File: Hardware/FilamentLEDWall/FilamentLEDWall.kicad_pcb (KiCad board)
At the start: 2 copper layers, 23 parts, among them U1 AMS1117-3.3, U2 AMS1117-5.0, U3 JXI5020GF

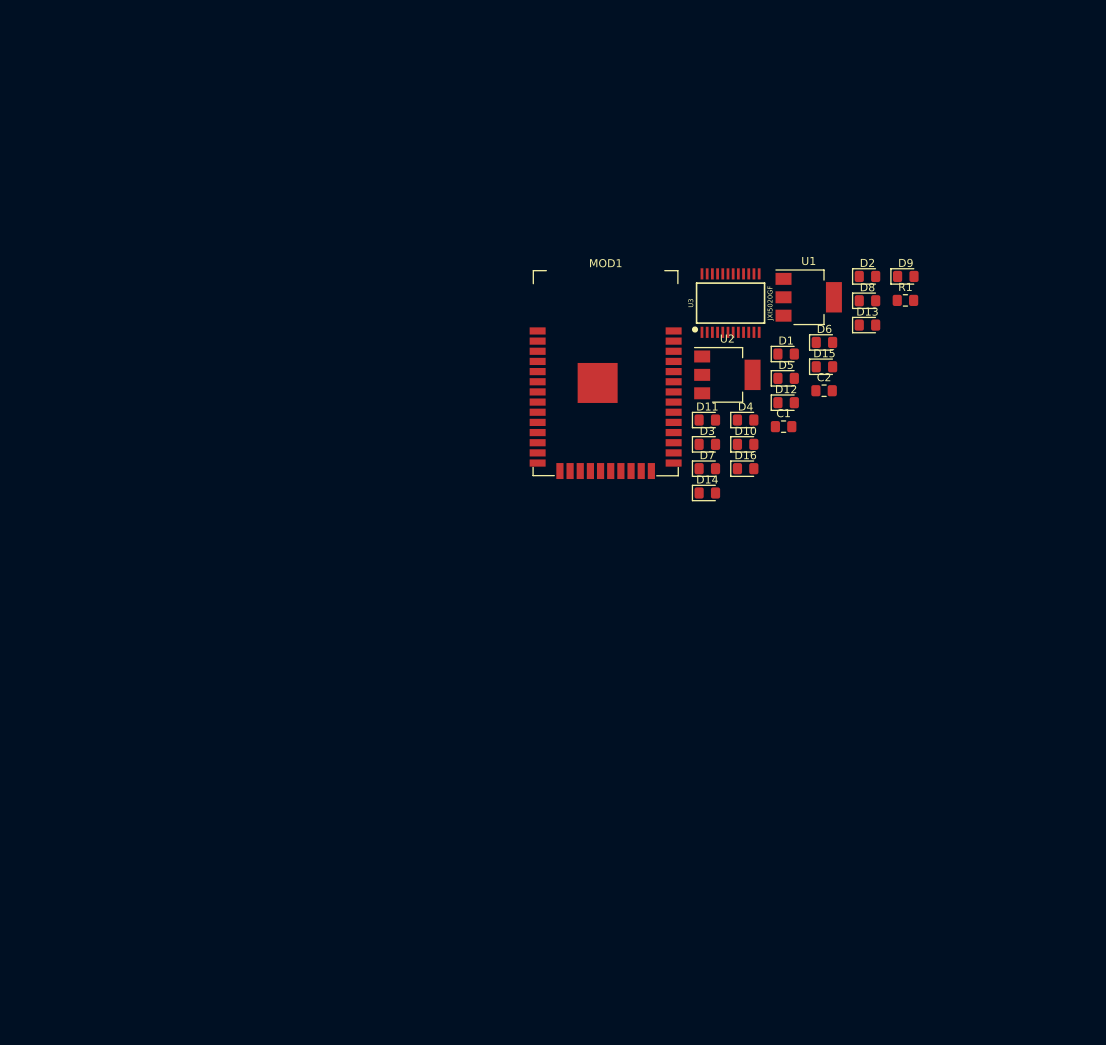
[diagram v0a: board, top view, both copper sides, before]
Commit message: updated circuit
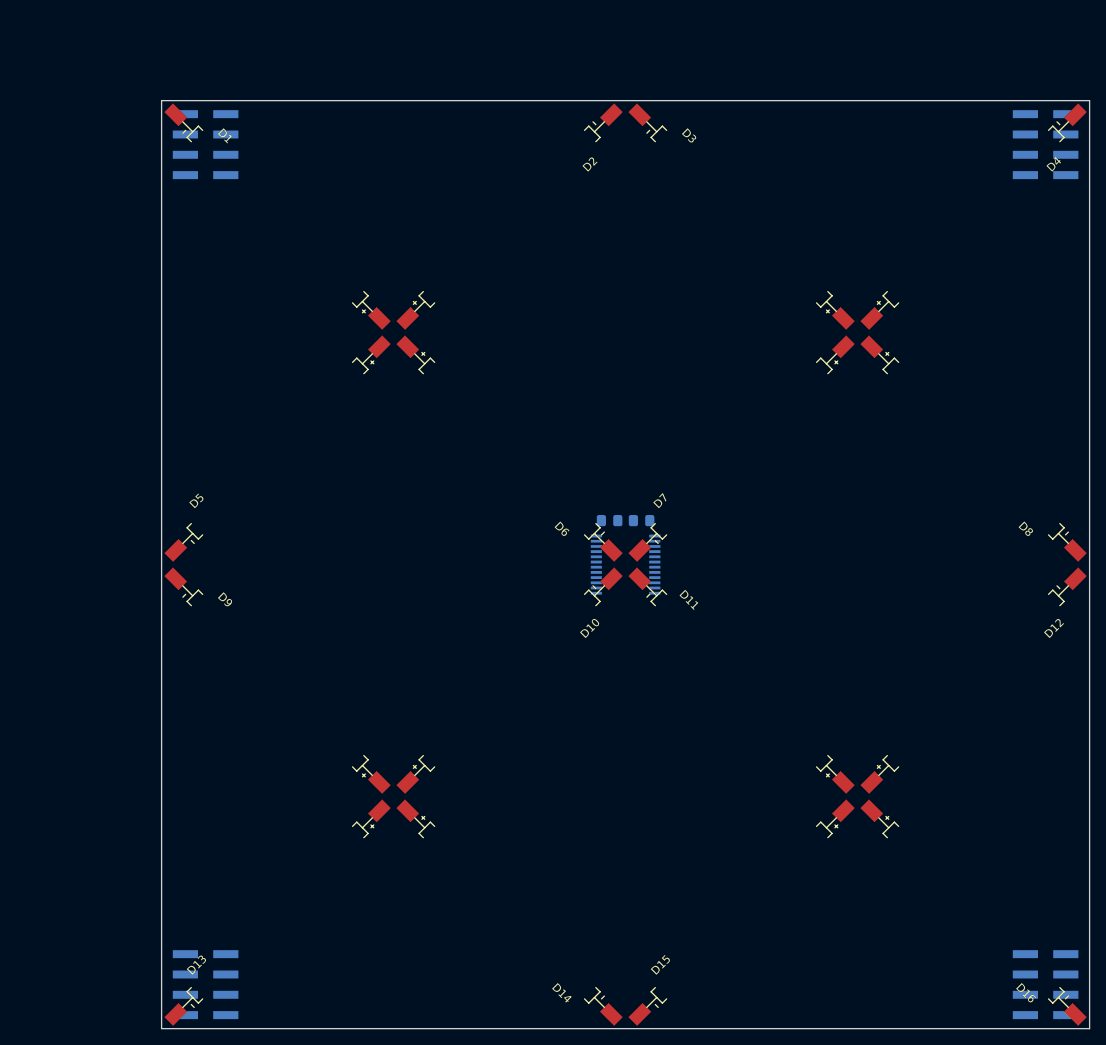
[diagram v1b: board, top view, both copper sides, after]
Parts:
- removed C2: 10uF, Capacitor_SMD:C_0805_2012Metric_Pad1.15x1.40mm_HandSolder
- removed MOD1: ESP32-WROOM-32, digikey-footprints:ESP32-WROOM-32D
- removed U1: AMS1117-3.3, Package_TO_SOT_SMD:SOT-223-3_TabPin2
- removed U2: AMS1117-5.0, Package_TO_SOT_SMD:SOT-223-3_TabPin2
- added J1: TopLeftConnector, Connector_PinHeader_2.54mm:PinHeader_2x04_P2.54mm_Vertical_SMD, B.Cu at (81.8, 40.0)
- added J2: TopLeftConnector, Connector_PinHeader_2.54mm:PinHeader_2x04_P2.54mm_Vertical_SMD, B.Cu at (81.8, 145.0)
- added J3: TopLeftConnector, Connector_PinHeader_2.54mm:PinHeader_2x04_P2.54mm_Vertical_SMD, B.Cu at (186.8, 145.0)
- added J4: TopLeftConnector, Connector_PinHeader_2.54mm:PinHeader_2x04_P2.54mm_Vertical_SMD, B.Cu at (186.8, 40.0)
- C1, R1, U3: moved to B.Cu
- D1, D10, D11, D12, D13, D14, D15, D16, D2, D3, D4, D5, D6, D7, D8, D9: footprint LED_SMD:LED_0805_2012Metric_Pad1.15x1.40mm_HandSolder -> FilamentLEDWall:FilamentLED_30mm
- moved D13 104.1 mm to (90.8, 136.0), turned to 315 degrees
- moved D9 93.4 mm to (90.8, 107.0), turned to 225 degrees
- moved D15 69.0 mm to (148.8, 136.0), turned to 315 degrees
- moved D1 65.8 mm to (90.8, 49.0), turned to 225 degrees
- moved D5 64.2 mm to (90.8, 78.0), turned to 315 degrees
- moved D16 62.4 mm to (177.8, 136.0), turned to 45 degrees
- moved D14 58.0 mm to (119.8, 136.0), turned to 45 degrees
- moved R1 46.1 mm to (132.2, 87.0)
- moved D2 45.4 mm to (119.8, 49.0), turned to 135 degrees
- moved D12 41.9 mm to (177.8, 107.0), turned to 135 degrees
- moved D10 41.7 mm to (119.8, 107.0), turned to 135 degrees
- moved D6 41.5 mm to (119.8, 78.0), turned to 45 degrees
- moved D4 38.2 mm to (177.8, 49.0), turned to 135 degrees
- moved U3 35.2 mm to (134.2, 92.5), turned to 270 degrees
- moved D11 32.9 mm to (148.8, 107.0), turned to 225 degrees
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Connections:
- C1 pad 1: /3.3V_MCU -> /5V_LED
- U3 pad 22: (no net) -> LED_SDO
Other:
- board outline added: 116 x 116 mm
- rule pad_to_mask_clearance: 0.051 -> 0.05

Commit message: Updated light PCB v0.1
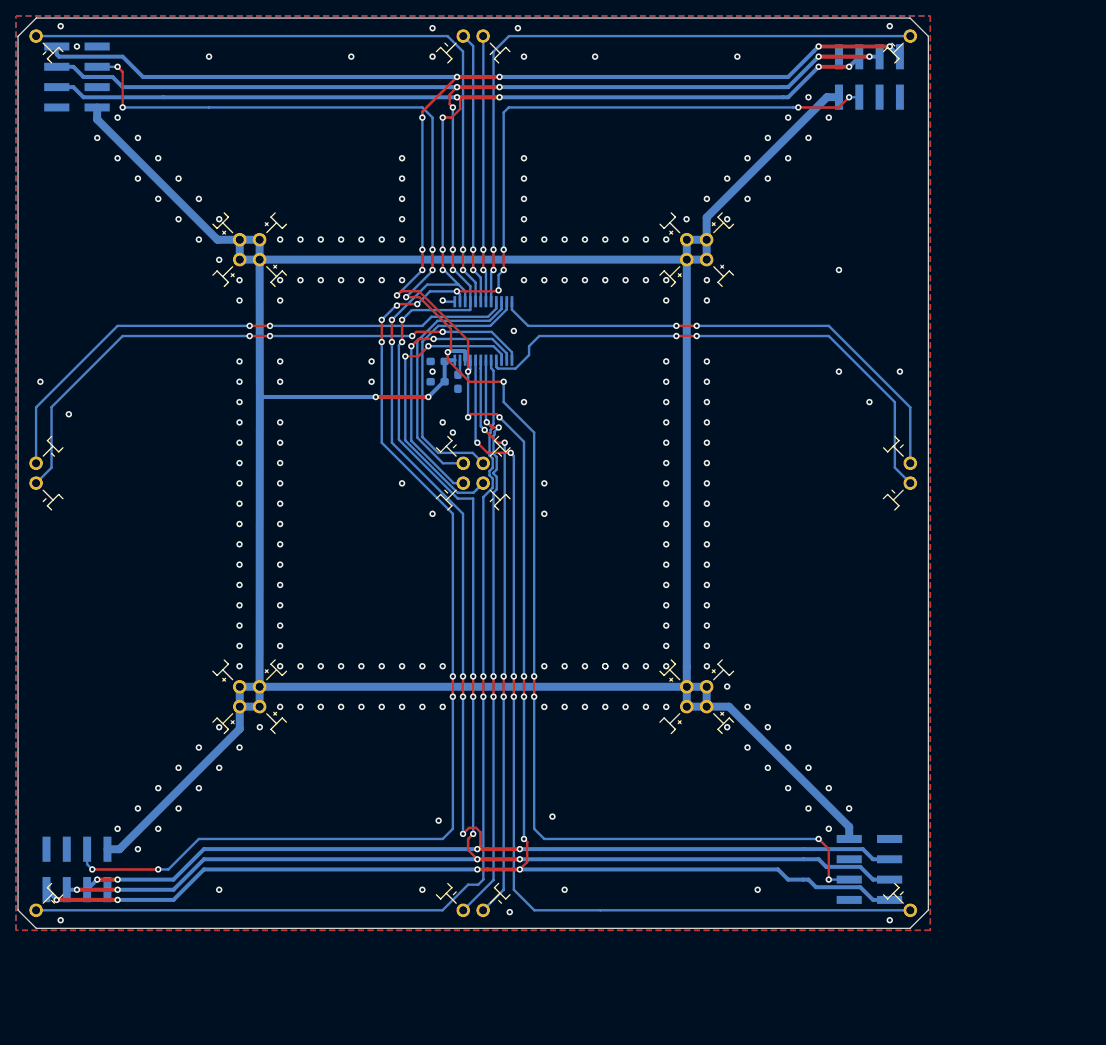
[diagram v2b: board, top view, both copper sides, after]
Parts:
- added C2: 100nF, Capacitor_SMD:C_0603_1608Metric_Pad1.05x0.95mm_HandSolder, B.Cu at (110.8, 67.1)
- C1: footprint Capacitor_SMD:C_0805_2012Metric_Pad1.15x1.40mm_HandSolder -> Capacitor_SMD:C_0603_1608Metric_Pad1.05x0.95mm_HandSolder
- J2: value TopLeftConnector -> BottomLeftConnector
- J3: value TopLeftConnector -> BottomRightConnector
- J4: value TopLeftConnector -> TopRightConnector
- R1: footprint Resistor_SMD:R_0805_2012Metric_Pad1.15x1.40mm_HandSolder -> Resistor_SMD:R_0603_1608Metric_Pad1.05x0.95mm_HandSolder
- moved U3 34.2 mm to (116.5, 63.3), turned to 0 degrees
- moved C1 30.8 mm to (110.8, 69.6), turned to 180 degrees
- moved J3 26.3 mm to (164.7, 130.6), turned to 180 degrees
- moved R1 25.7 mm to (113.3, 69.6), turned to 270 degrees
- moved D16 24.4 mm to (157.1, 123.0)
- moved D12 23.9 mm to (157.1, 95.0)
- moved J4 23.6 mm to (164.7, 31.5), turned to 270 degrees
- moved D15 23.5 mm to (129.2, 123.0)
- moved D8 23.3 mm to (157.1, 67.1)
- moved D11 22.9 mm to (129.2, 95.0)
- moved D4 22.9 mm to (157.1, 39.2)
- moved D14 22.6 mm to (101.2, 123.0)
- moved D7 22.4 mm to (129.2, 67.1)
- moved D10 22.0 mm to (101.2, 95.0)
- moved D3 21.9 mm to (129.2, 39.2)
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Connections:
- D1 pad 2: 5V -> /5V_LED
- D10 pad 2: 5V -> /5V_LED
- D11 pad 2: 5V -> /5V_LED
- D12 pad 2: 5V -> /5V_LED
- D13 pad 2: 5V -> /5V_LED
- D14 pad 2: 5V -> /5V_LED
- D15 pad 2: 5V -> /5V_LED
- D16 pad 2: 5V -> /5V_LED
- D2 pad 2: 5V -> /5V_LED
- D3 pad 2: 5V -> /5V_LED
- D4 pad 2: 5V -> /5V_LED
- D5 pad 2: 5V -> /5V_LED
- D6 pad 2: 5V -> /5V_LED
- D7 pad 2: 5V -> /5V_LED
- D8 pad 2: 5V -> /5V_LED
- D9 pad 2: 5V -> /5V_LED
- J1 pad 2: LED_CLK -> /5V_LED
- J1 pad 3: LED_LE -> LED_CLK
- J1 pad 4: LED_OE -> (no net)
- J1 pad 5: GND -> LED_LE
- J1 pad 7: LED_SDI -> LED_OE
- J1 pad 8: /5V_LED -> GND
- J2 pad 2: LED_CLK -> /5V_LED
- J2 pad 3: LED_LE -> LED_CLK
- J2 pad 4: LED_OE -> LED_SDI
- J2 pad 5: GND -> LED_LE
- J2 pad 6: LED_SDO -> (no net)
- J2 pad 7: LED_SDI -> LED_OE
- J2 pad 8: /5V_LED -> GND
- J3 pad 2: LED_CLK -> /5V_LED
- J3 pad 3: LED_LE -> LED_CLK
- J3 pad 4: LED_OE -> (no net)
- J3 pad 5: GND -> LED_LE
- J3 pad 7: LED_SDI -> LED_OE
- J3 pad 8: /5V_LED -> GND
- J4 pad 2: LED_CLK -> /5V_LED
- J4 pad 3: LED_LE -> LED_CLK
- J4 pad 4: LED_OE -> LED_SDI
- J4 pad 5: GND -> LED_LE
- J4 pad 6: LED_SDO -> (no net)
- J4 pad 7: LED_SDI -> LED_OE
- J4 pad 8: /5V_LED -> GND
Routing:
- net /5V_LED: track 0.00 -> 383.3 mm, vias 0 -> 2
- net LED_OE: track 0.00 -> 334.6 mm, vias 0 -> 18
- net LED_LE: track 0.00 -> 322.7 mm, vias 0 -> 16
- net LED_CLK: track 0.00 -> 317.5 mm, vias 0 -> 16
- net LED_SDI: track 0.00 -> 202.6 mm, vias 0 -> 14
- net LED_SDO: track 0.00 -> 195.4 mm, vias 0 -> 11
- net OUT12: track 0.00 -> 123.7 mm, vias 0 -> 2
- net OUT15: track 0.00 -> 120.5 mm, vias 0 -> 4
- net OUT0: track 0.00 -> 86.1 mm, vias 0 -> 2
- net OUT3: track 0.00 -> 84.3 mm, vias 0 -> 2
- net OUT8: track 0.00 -> 73.8 mm, vias 0 -> 4
- net OUT13: track 0.00 -> 72.4 mm, vias 0 -> 4
- net OUT14: track 0.00 -> 71.7 mm, vias 0 -> 4
- net OUT4: track 0.00 -> 70.5 mm, vias 0 -> 2
- net OUT11: track 0.00 -> 67.4 mm, vias 0 -> 2
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- added copper zone on B.Cu, net GND
- added copper zone on F.Cu, net GND
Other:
- board size 116 x 116 mm -> 113.8 x 113.8 mm
- board text added: "100nF"
- board text added: "10uF"
- board text added: "Filament Wall Cell v0.1 Sandbox Workshop Designed by Caorx Wangyw"
- board text added: "INPUT"
- board text added: "Iout=Vext(1.24V)/Rext*15"
- board text added: "OUTPUT"
- board text added: "R_EXT"
